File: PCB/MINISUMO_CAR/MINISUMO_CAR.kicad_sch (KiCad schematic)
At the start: 12 parts, among them U1 XY-XHB2.54-4A11, U2 XY-XHB2.54-4A11, U3 XY-XHB2.54-4A11, U4 XY-XHB2.54-4A11, U5 XY-XHB2.54-3A11, U6 XY-XHB2.54-3A11

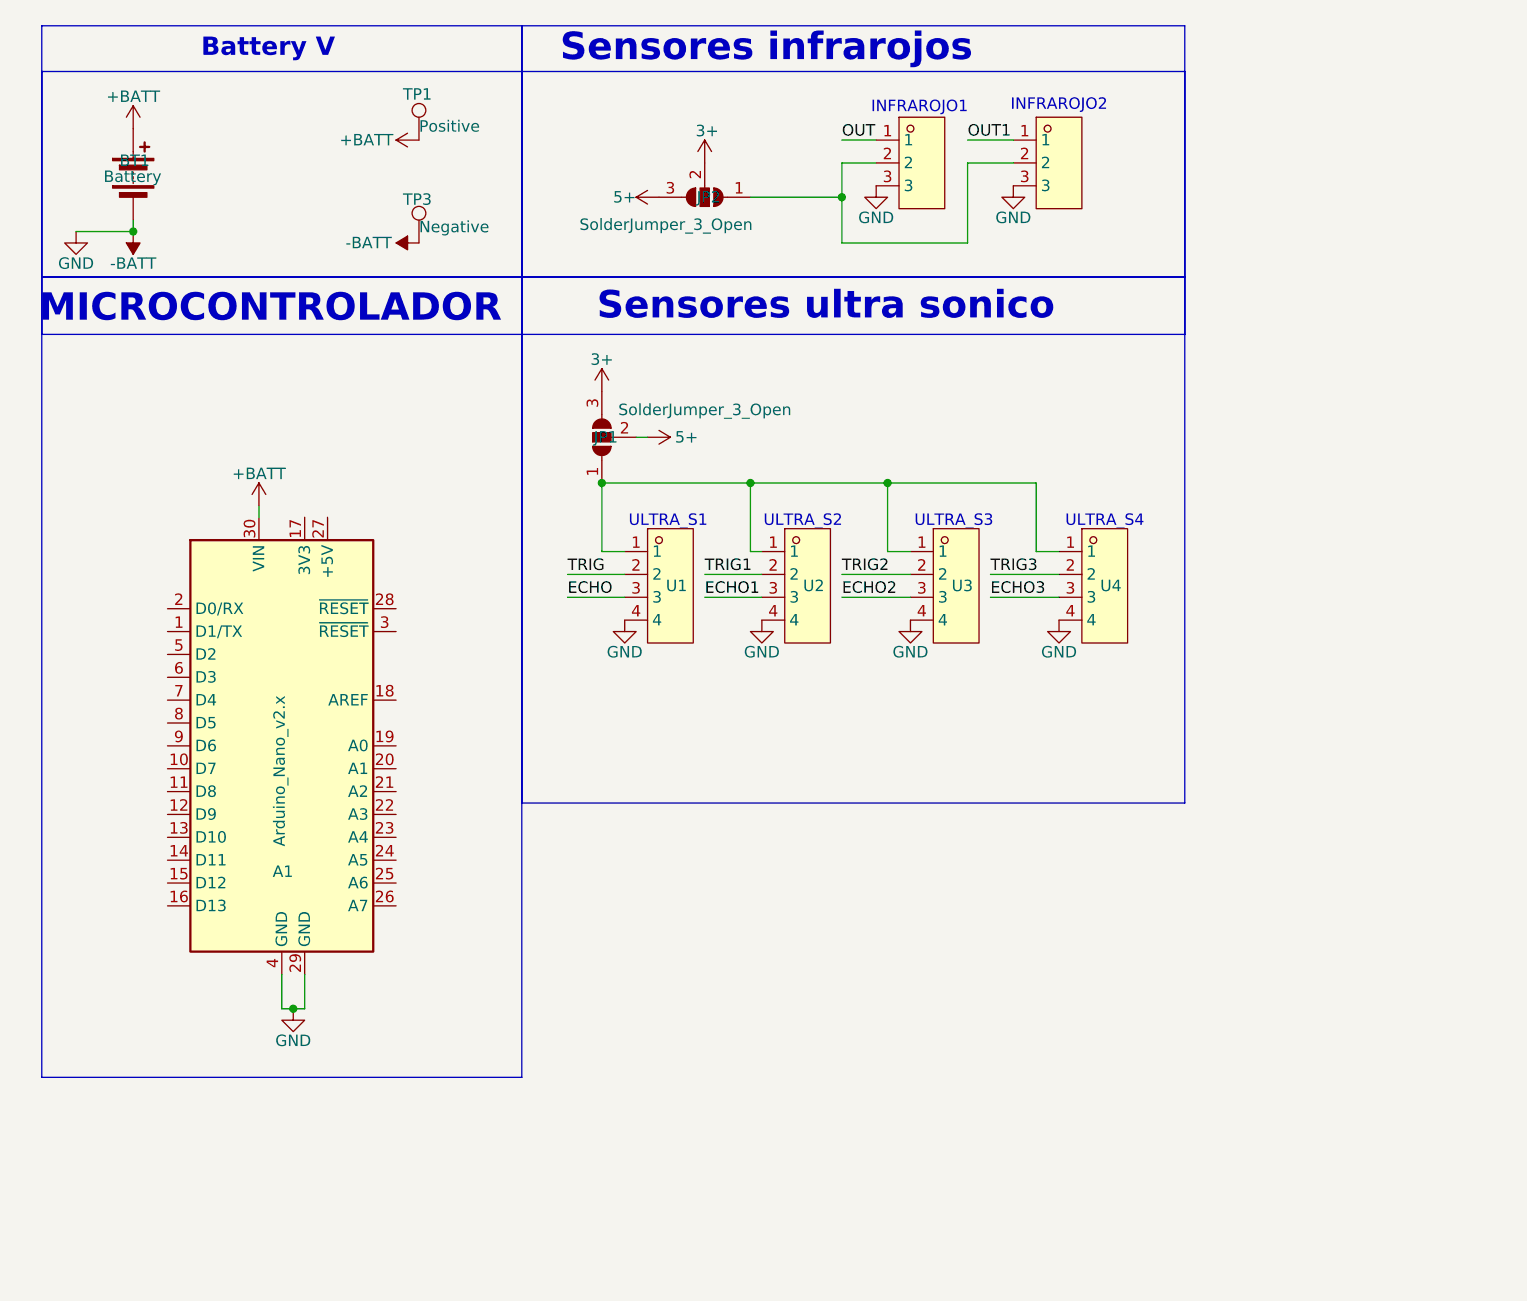
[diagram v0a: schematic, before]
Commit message: add push init and driver H
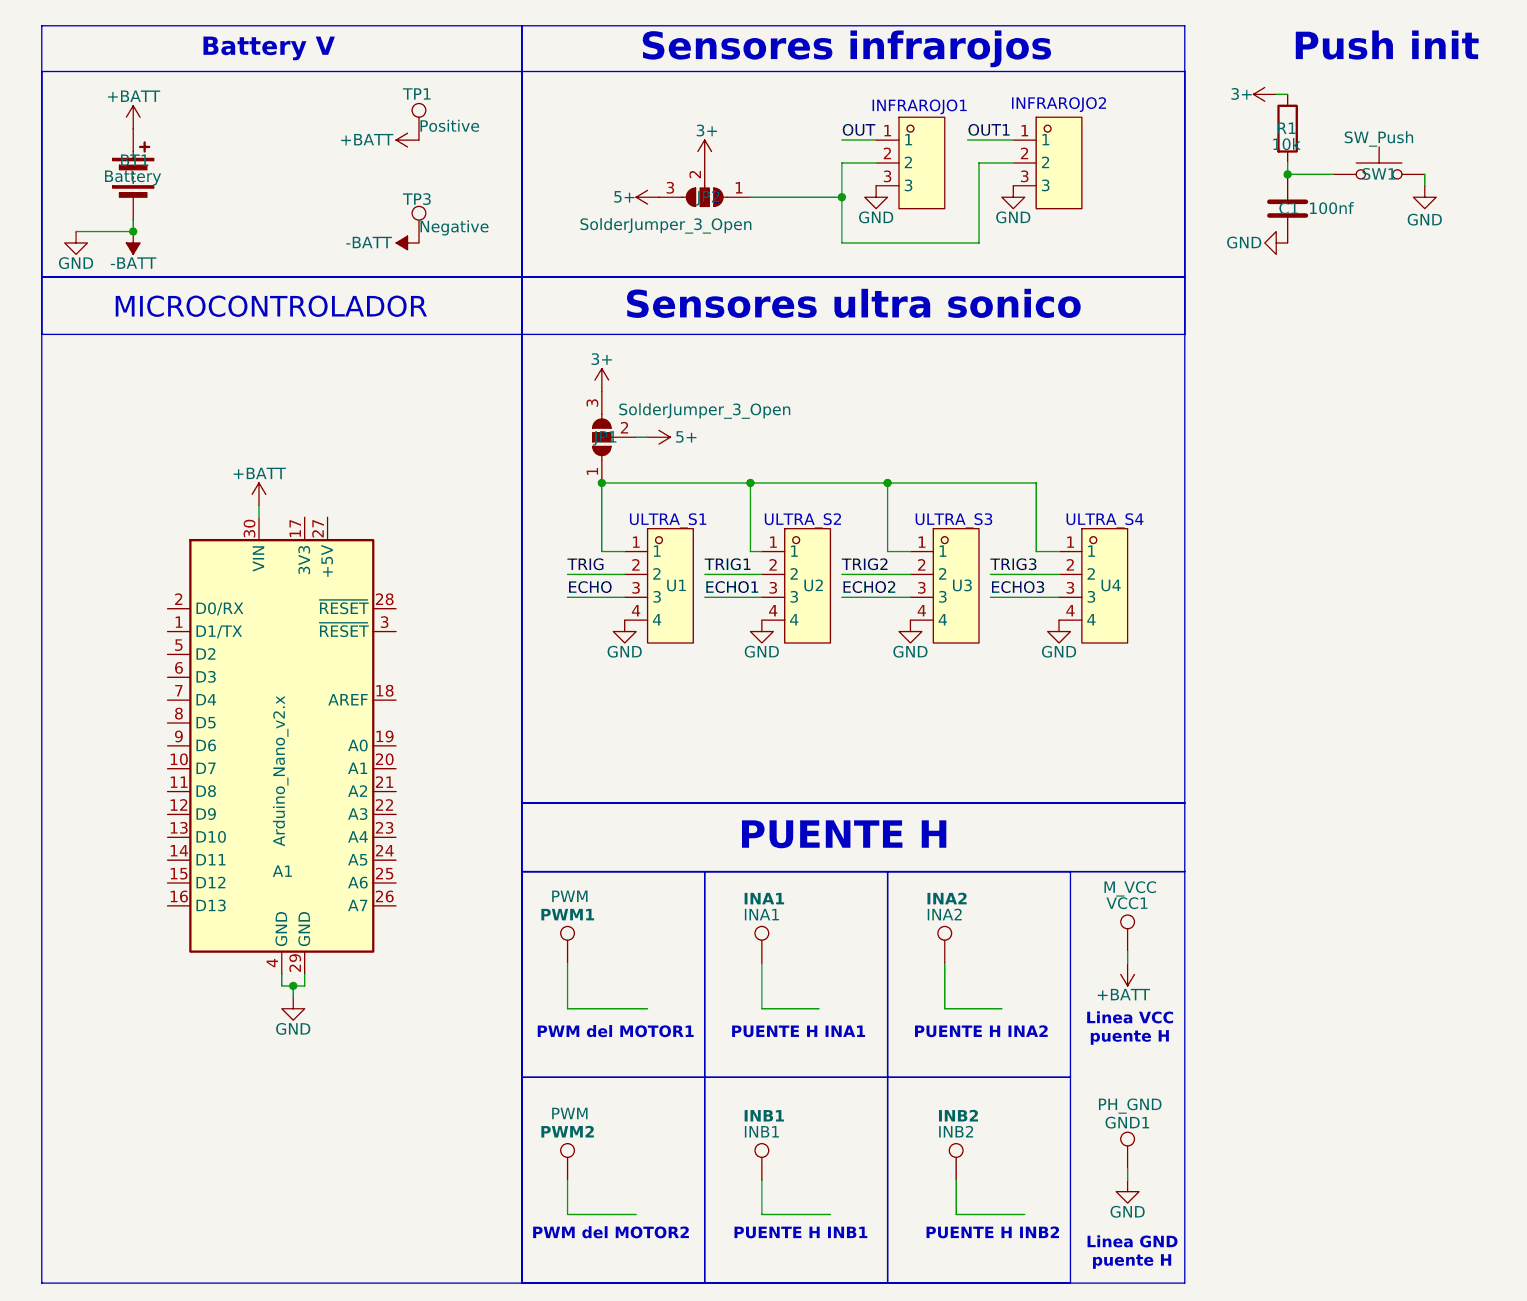
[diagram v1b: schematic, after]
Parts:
- added C1: 100nf, symbol Device:C
- added GND1: PH_GND, Connector_PinHeader_2.00mm:PinHeader_1x01_P2.00mm_Vertical, symbol Connector:TestPoint
- added INA1: INA1, Connector_PinHeader_2.00mm:PinHeader_1x01_P2.00mm_Vertical, symbol Connector:TestPoint
- added INA2: INA2, Connector_PinHeader_2.00mm:PinHeader_1x01_P2.00mm_Vertical, symbol Connector:TestPoint
- added INB1: INB1, Connector_PinHeader_2.00mm:PinHeader_1x01_P2.00mm_Vertical, symbol Connector:TestPoint
- added INB2: INB2, Connector_PinHeader_2.00mm:PinHeader_1x01_P2.00mm_Vertical, symbol Connector:TestPoint
- added PWM1, PWM2: PWM, Connector_PinHeader_2.00mm:PinHeader_1x01_P2.00mm_Vertical, symbol Connector:TestPoint
- added R1: 10k, symbol Device:R
- added SW1: SW_Push, symbol Switch:SW_Push
- added VCC1: M_VCC, Connector_PinHeader_2.00mm:PinHeader_1x01_P2.00mm_Vertical, symbol Connector:TestPoint
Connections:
- net +BATT: now also VCC1.1
- net -BATT: now also C1.2, GND1.1, SW1.2
- net 3+: now also R1.1
- new net: C1.1, R1.2, SW1.1
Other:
- note added: "Linea GND puente H"
- note added: "Linea VCC puente H"
- note added: "PUENTE H"
- note added: "PUENTE H INA1"
- note added: "PUENTE H INA2"
- note added: "PUENTE H INB1"
- note added: "PUENTE H INB2"
- note added: "PWM del MOTOR1"
- note added: "PWM del MOTOR2"
- note added: "Push init"

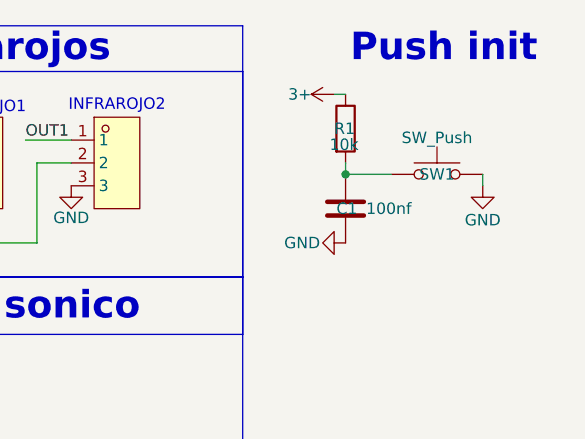
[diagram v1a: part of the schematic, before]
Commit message: Finish to day 7_27_2026
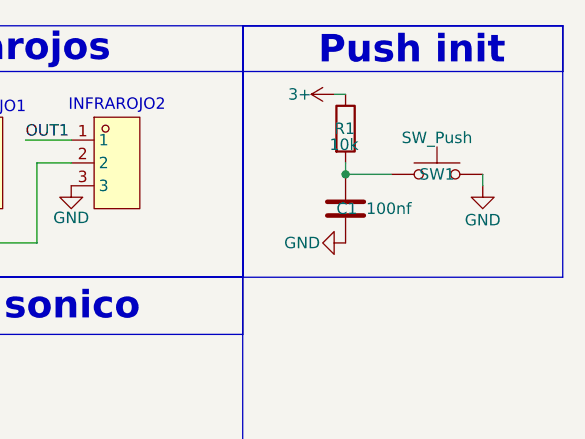
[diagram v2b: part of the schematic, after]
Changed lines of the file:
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@@
+	)
+	(rectangle
+		(start 142.24 16.51)
+		(end 177.8 21.59)
+		(stroke
+			(width 0)
+			(type default)
+		)
+		(fill
+			(type none)
+		)
 	)
 	(rectangle
@@
 	)
 	(rectangle
+		(start 142.24 16.51)
+		(end 177.8 44.45)
+		(stroke
+			(width 0)
+			(type default)
+		)
+		(fill
+			(type none)
+		)
+	)
+	(rectangle
 		(start 68.58 44.45)
 		(end 142.24 102.87)
@@
 	(text "Push init"
 		(exclude_from_sim no)
-		(at 164.592 19.05 0)
-		(effects
-			(font
+		(at 161.036 19.304 0)
+		(effects
+			(font
